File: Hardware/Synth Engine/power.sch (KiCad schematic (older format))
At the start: 9 parts, among them J1 Barrel_Jack, U4 TL074, U7 V7805-1000

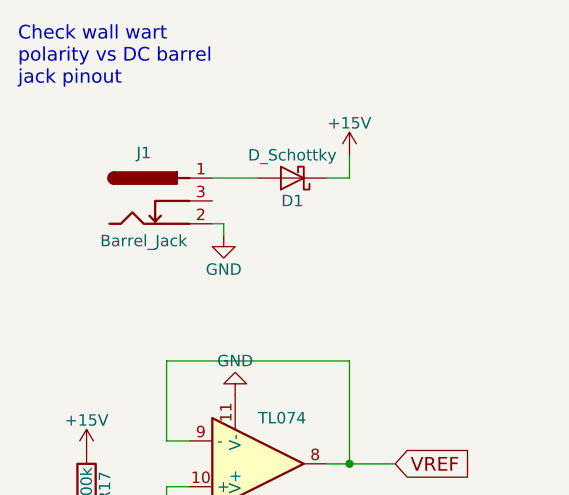
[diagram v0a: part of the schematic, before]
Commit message: new release candidate. Passes DRC.
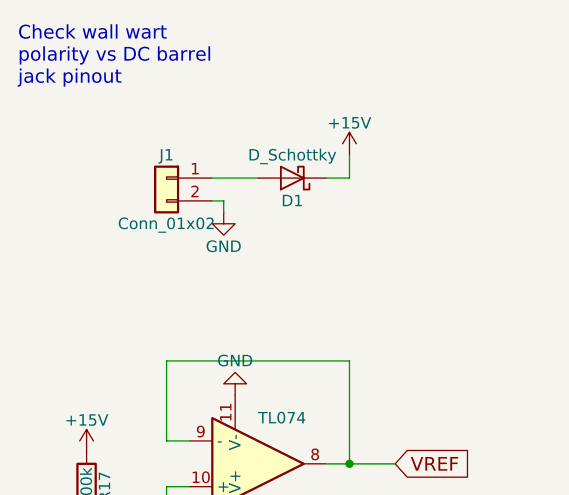
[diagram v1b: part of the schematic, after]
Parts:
- removed J1: Barrel_Jack, Connectors:BARREL_JACK, symbol Barrel_Jack
- added J1: Conn_01x02, Connectors_Molex:Molex_KK-6410-02_02x2.54mm_Straight, symbol Conn_01x02
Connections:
- net GND: now also J1.2 (Pin_2)
- net at D1.2 (A): now also J1.1 (Pin_1)
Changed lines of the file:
@@
 $EndDescr
-$Comp
-L Barrel_Jack J1
-U 1 1 5C392266
-P 1800 1700
-F 0 "J1" H 1800 1910 50  0000 C CNN
-F 1 "Barrel_Jack" H 1800 1525 50  0000 C CNN
-F 2 "Connectors:BARREL_JACK" H 1850 1660 50  0001 C CNN
-F 3 "" H 1850 1660 50  0001 C CNN
-	1    1800 1700
-	1    0    0    -1
-$EndComp
 $Comp
 L +15V #PWR017
@@
 L GND #PWR018
 U 1 1 5C39231B
-P 2150 1850
-F 0 "#PWR018" H 2150 1600 50  0001 C CNN
-F 1 "GND" H 2150 1700 50  0000 C CNN
-F 2 "" H 2150 1850 50  0001 C CNN
-F 3 "" H 2150 1850 50  0001 C CNN
-	1    2150 1850
-	1    0    0    -1
-$EndComp
-Wire Wire Line
-	2150 1850 2150 1800
-Wire Wire Line
-	2150 1800 2100 1800
+P 2150 1750
+F 0 "#PWR018" H 2150 1500 50  0001 C CNN
+F 1 "GND" H 2150 1600 50  0000 C CNN
+F 2 "" H 2150 1750 50  0001 C CNN
+F 3 "" H 2150 1750 50  0001 C CNN
+	1    2150 1750
+	1    0    0    -1
+$EndComp
+Wire Wire Line
+	2150 1750 2150 1700
+Wire Wire Line
+	2150 1700 2100 1700
 Wire Wire Line
 	2700 1500 2700 1600
@@
 $EndComp
 Connection ~ 5950 2750
+$Comp
+L Conn_01x02 J1
+U 1 1 5C75C161
+P 1900 1600
+F 0 "J1" H 1900 1700 50  0000 C CNN
+F 1 "Conn_01x02" H 1900 1400 50  0000 C CNN
+F 2 "Connectors_Molex:Molex_KK-6410-02_02x2.54mm_Straight" H 1900 1600 50  0001 C CNN
+F 3 "" H 1900 1600 50  0001 C CNN
+	1    1900 1600
+	-1   0    0    -1
+$EndComp
 $EndSCHEMATC
